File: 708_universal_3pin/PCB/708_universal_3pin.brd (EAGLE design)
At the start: 27.9 x 39.4 mm, 17 parts

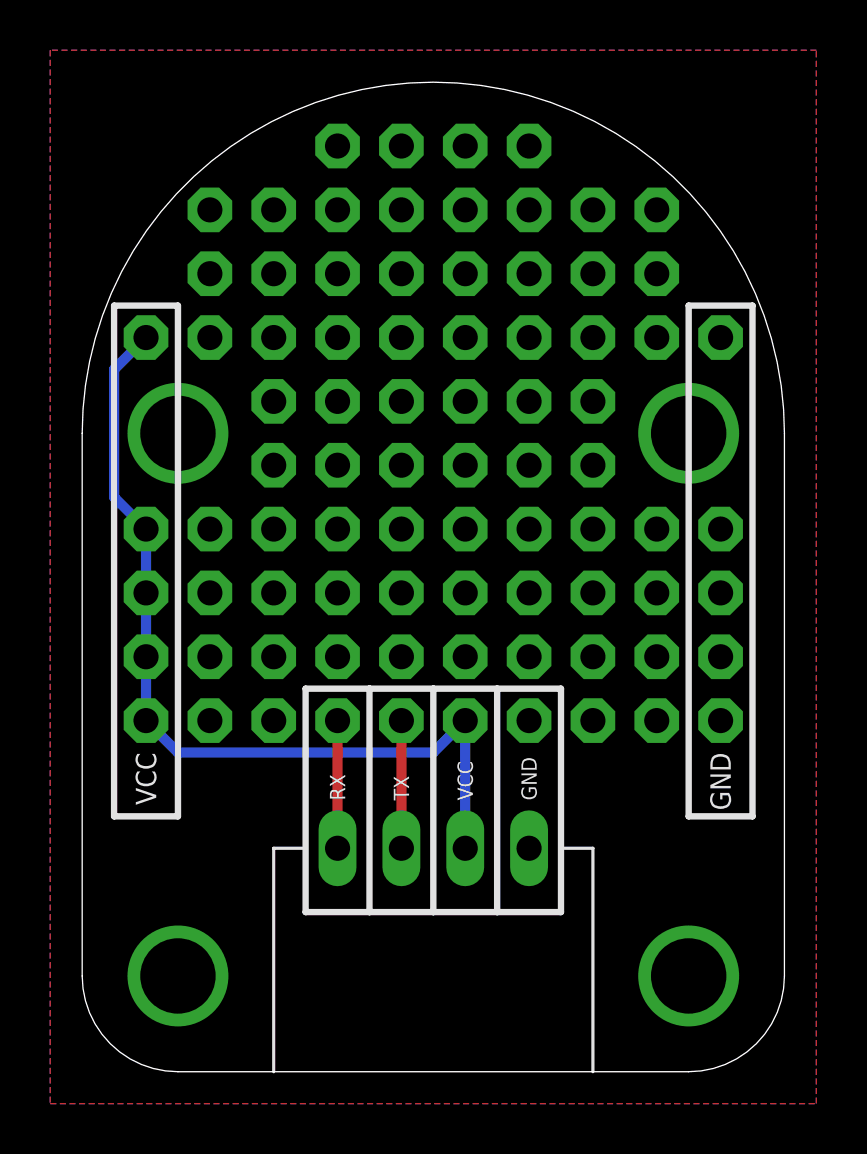
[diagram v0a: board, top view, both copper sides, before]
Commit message: rename prod-number directory change breakout layout
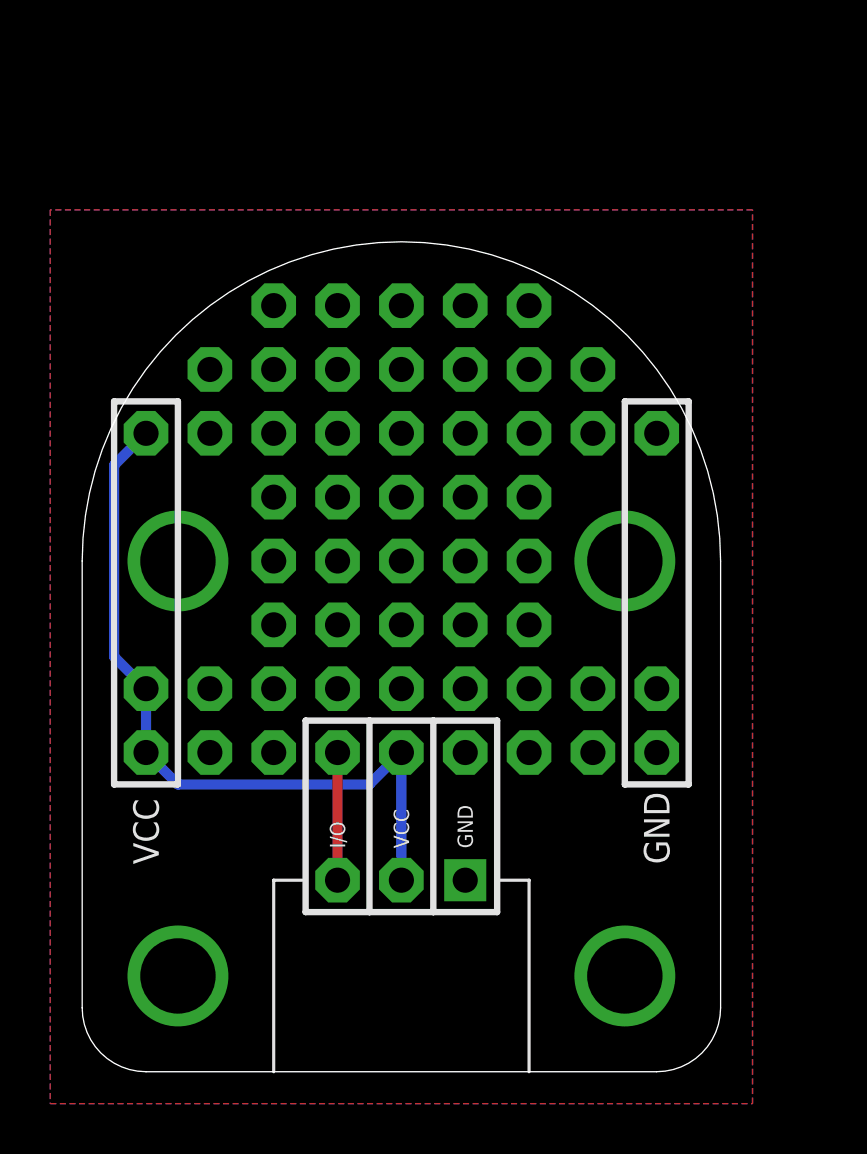
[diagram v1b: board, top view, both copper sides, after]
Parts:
- removed J11, J12, J13, J14, J15: (no value), FaBo-etc:PIN_1X1_NONAME
- J1: device FaBo-Template:FABO_BRICK_SERIAL_UNIVERSAL -> FaBo-Template:FABO_BRICK_3PIN_UNIVERSAL
- moved J9 24.7 mm to (22.9, 15.2)
- moved J8 22.2 mm to (22.9, 12.7)
- moved J7 14.2 mm to (15.2, 12.7)
- moved J4 12.8 mm to (2.54, 12.7)
- moved J6 8.89 mm to (2.54, 25.4)
- moved J10 4.58 mm to (22.9, 25.4)
- moved J1 2.84 mm to (12.7, 16.5)
- moved J2 1.27 mm to (10.2, 12.7)
- moved J3 1.27 mm to (12.7, 12.7)
- moved U$3 1.27 mm to (12.7, 2.54)
- moved J5 1.27 mm to (2.54, 15.2)
- renumbered U$2 to U$1
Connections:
- removed net RX: J1.RX, J2.1
- removed net TX: J1.TX, J3.1
- new net IO: J1.IN/OUT, J2.1
- net GND: now also J7.1, J8.1, J9.1; no longer J11.1, J12.1, J13.1, J14.1, J15.1
- net VCC: now also J3.1; no longer J7.1, J8.1, J9.1
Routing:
- net VCC: track 35.1 -> 30.0 mm
- net TX: track 5.08 -> 0.00 mm
- net RX: track 5.08 -> 0.00 mm
- net IO: track 0.00 -> 5.08 mm
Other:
- board size 27.9 x 39.4 mm -> 25.4 x 33 mm
- board text added: "#708"
- board text added: "Rev.1.0.2"
- board text removed: "#702"
- board text removed: "Rev.1.0.1"
